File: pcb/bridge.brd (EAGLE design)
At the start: 104.2 x 63.6 mm, 29 parts, among them IC1 ARDUINO_PRO_MICRO, IC2 LM358D, X1 SZARKBUS, X2 RSENSE, X3 +12V

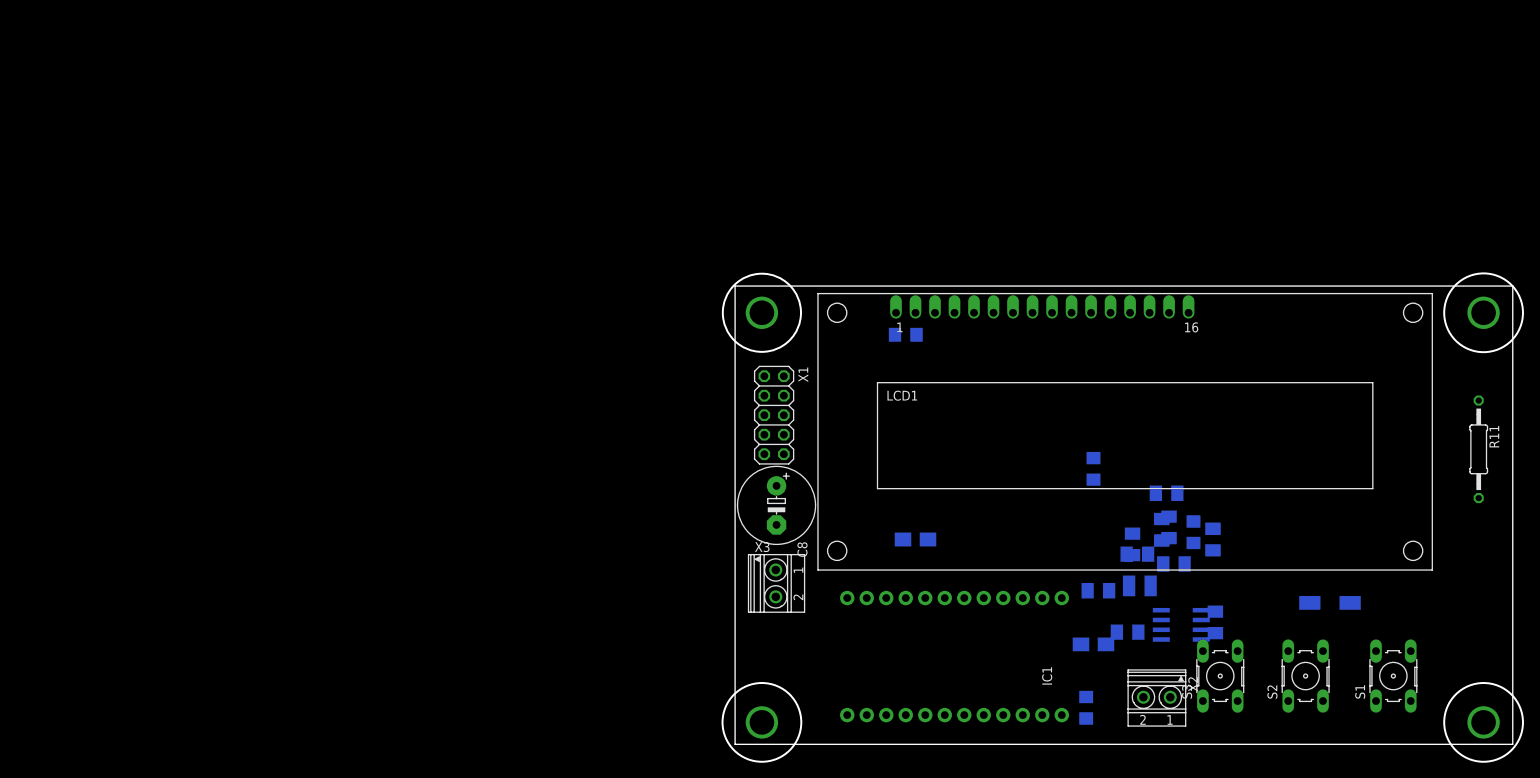
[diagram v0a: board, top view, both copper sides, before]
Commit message: bridge: board shape.
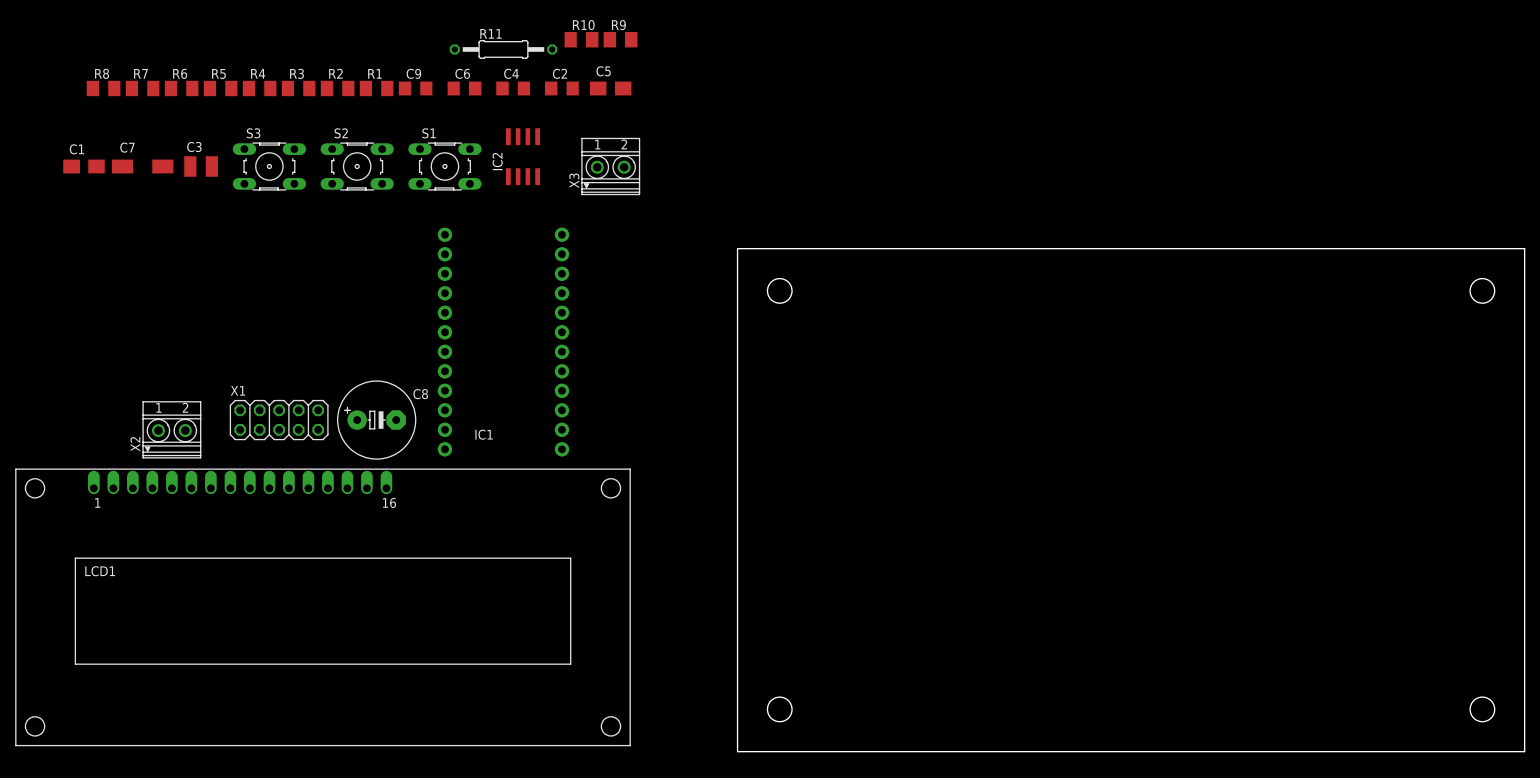
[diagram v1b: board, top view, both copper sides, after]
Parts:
- moved C7 164.7 mm to (-77.5, 76.2), flipped to the top
- moved R7 151.3 mm to (-77.5, 86.4), flipped to the top, turned to 0 degrees
- moved R8 146.6 mm to (-82.5, 86.4), flipped to the top, turned to 0 degrees
- moved R6 143.3 mm to (-72.4, 86.4), flipped to the top
- moved S3 140.5 mm to (-61.0, 76.2), turned to 0 degrees
- moved S2 140.2 mm to (-49.5, 76.2), turned to 0 degrees
- moved S1 140.2 mm to (-38.1, 76.2), turned to 0 degrees
- moved R3 138.2 mm to (-57.1, 86.4), flipped to the top, turned to 0 degrees
- moved R11 137.3 mm to (-30.5, 91.4), turned to 0 degrees
- moved R5 134.0 mm to (-67.3, 86.4), flipped to the top
- moved C3 133.9 mm to (-69.8, 76.2), flipped to the top, turned to 0 degrees
- moved X2 132.9 mm to (-73.7, 41.9), turned to 0 degrees
- moved R4 129.4 mm to (-62.2, 86.4), flipped to the top, turned to 0 degrees
- moved R1 120.7 mm to (-47.0, 86.4), flipped to the top, turned to 0 degrees
- moved R2 118.7 mm to (-52.1, 86.4), flipped to the top, turned to 0 degrees
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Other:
- board size 104.2 x 63.6 mm -> 102.5 x 65.5 mm
